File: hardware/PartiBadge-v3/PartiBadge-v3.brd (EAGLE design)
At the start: 118.9 x 117.7 mm, 26 parts, among them J1 I2C, J2 Supply, T1 MMBT4401-7-F

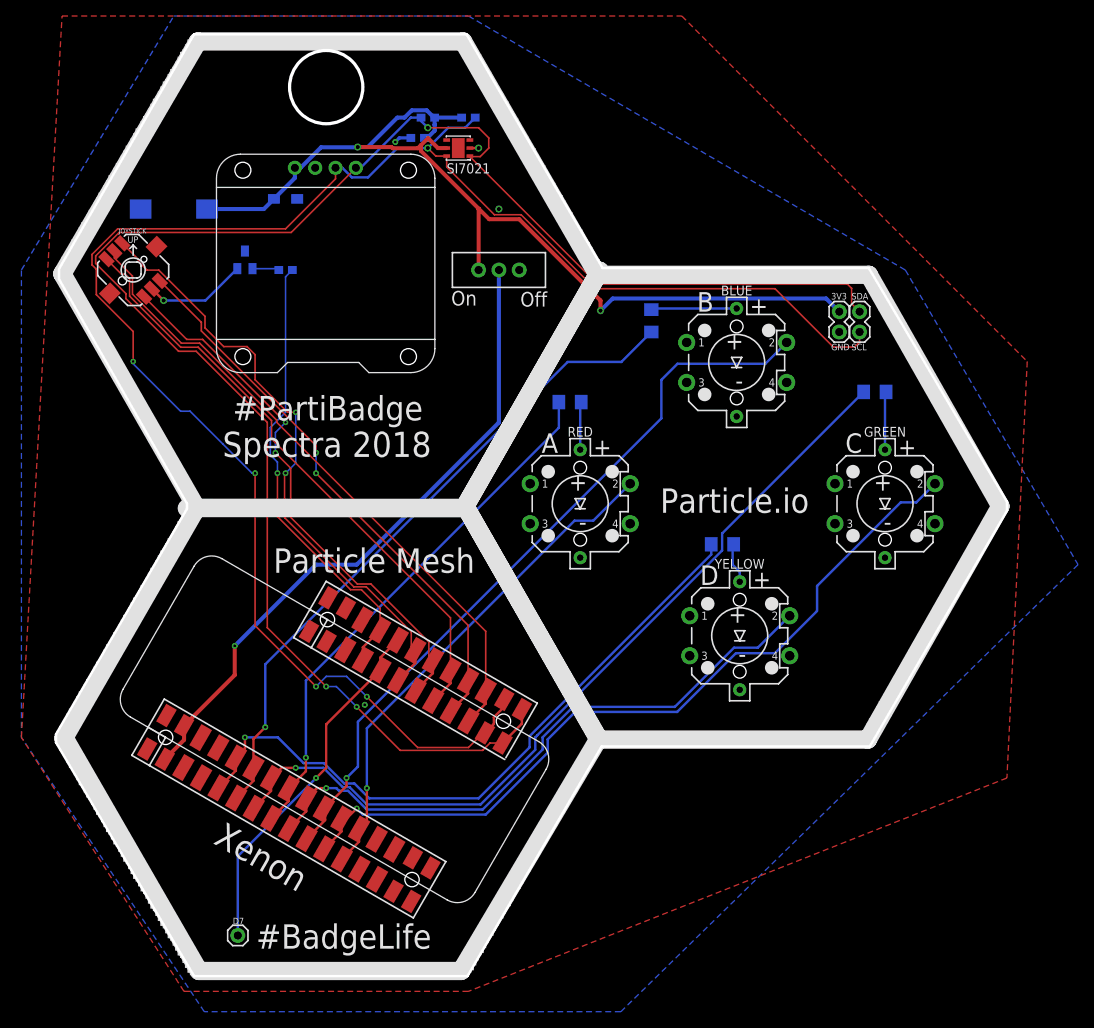
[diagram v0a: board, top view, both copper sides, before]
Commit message: finished Xenon port
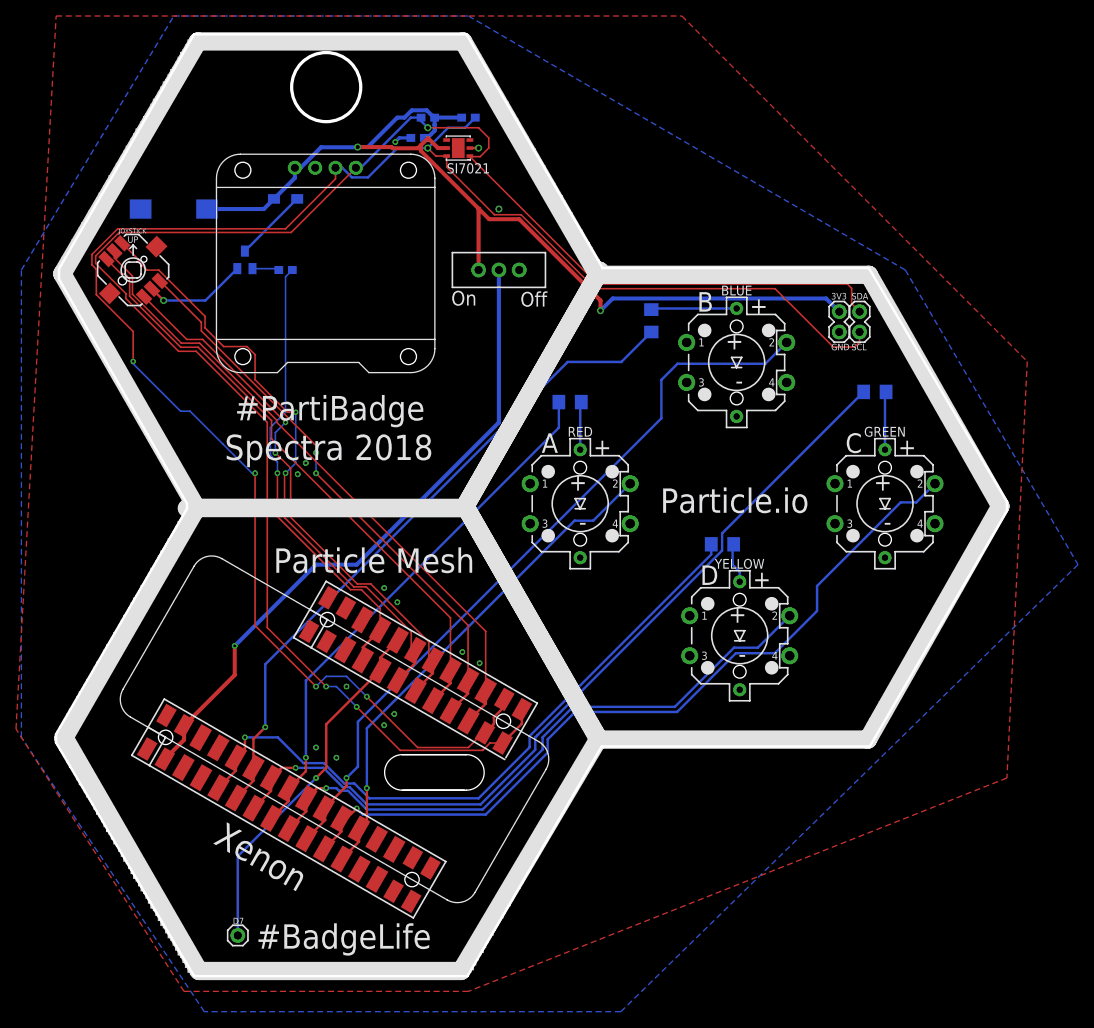
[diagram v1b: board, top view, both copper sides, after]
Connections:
- new net N$18: D1.A, T1.C
- net GND: no longer D1.A, T1.C
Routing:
- net N$18: track 0.00 -> 9.23 mm
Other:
- outline, holes or cut-outs redrawn
- board text added: "*NON PLATED * *SLOT*"
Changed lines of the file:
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@@
 <drawing>
 <settings>
-<setting alwaysvectorfont="no"/>
+<setting alwaysvectorfont="yes"/>
 <setting verticaltext="up"/>
 </settings>
-<grid distance="50" unitdist="mil" unit="mil" style="lines" multiple="1" display="no" altdistance="5" altunitdist="mil" altunit="mil"/>
+<grid distance="5" unitdist="mil" unit="mil" style="dots" multiple="1" display="yes" altdistance="5" altunitdist="mil" altunit="mil"/>
 <layers>
 <layer number="1" name="Top" color="4" fill="1" visible="yes" active="yes"/>
@@
 <layer number="26" name="bNames" color="7" fill="1" visible="yes" active="yes"/>
 <layer number="27" name="tValues" color="7" fill="1" visible="yes" active="yes"/>
-<layer number="28" name="bValues" color="7" fill="1" visible="yes" active="yes"/>
+<layer number="28" name="bValues" color="7" fill="1" visible="no" active="yes"/>
 <layer number="29" name="tStop" color="7" fill="3" visible="no" active="yes"/>
 <layer number="30" name="bStop" color="7" fill="6" visible="no" active="yes"/>
@@
 <layer number="45" name="Holes" color="7" fill="1" visible="yes" active="yes"/>
 <layer number="46" name="Milling" color="3" fill="1" visible="no" active="yes"/>
-<layer number="47" name="Measures" color="7" fill="1" visible="no" active="yes"/>
+<layer number="47" name="Measures" color="7" fill="1" visible="yes" active="yes"/>
 <layer number="48" name="Document" color="7" fill="1" visible="yes" active="yes"/>
 <layer number="49" name="Reference" color="7" fill="1" visible="yes" active="yes"/>
@@
 <wire x1="4.318" y1="33.401" x2="20.701" y2="61.595" width="0.3048" layer="20"/>
 <wire x1="20.701" y1="61.595" x2="20.701" y2="62.23" width="0.3048" layer="20"/>
-<text x="26.416" y="72.644" size="3.048" layer="21" font="vector" ratio="18">#PartiBadge</text>
-<text x="25.146" y="68.072" size="3.1496" layer="21" font="vector" ratio="18">Spectra 2018</text>
-<circle x="38.1" y="114.3" radius="4.57905" width="0.4064" layer="20"/>
+<text x="26.67" y="72.644" size="3.048" layer="21" font="vector" ratio="18">#PartiBadge</text>
+<text x="25.4" y="67.691" size="3.1496" layer="21" font="vector" ratio="18">Spectra 2018</text>
+<circle x="38.1" y="114.3" radius="4.318" width="0.4064" layer="20"/>
 <text x="65.024" y="68.58" size="2.4384" layer="21" font="vector" ratio="18">A</text>
 <text x="84.455" y="86.233" size="2.4384" layer="21" font="vector" ratio="18">B</text>
@@
 <rectangle x1="119.3546" y1="103.5812" x2="157.4546" y2="106.1212" layer="49"/>
 <rectangle x1="119.3546" y1="98.5012" x2="157.4546" y2="101.0412" layer="49"/>
-<dimension x1="2.54" y1="57.15" x2="104.14" y2="57.15" x3="53.34" y3="132.334" textsize="1.778" layer="47" dtype="diameter" unit="inch" visible="yes"/>
-<dimension x1="48.76095" y1="101.6" x2="57.91905" y2="101.6" x3="53.34" y3="124.46" textsize="1.778" layer="47" dtype="diameter" unit="inch" visible="yes"/>
 <dimension x1="51.689" y1="83.058" x2="64.008" y2="83.058" x3="57.8485" y3="111.125" textsize="1.778" layer="47" visible="yes"/>
-<dimension x1="61.71543125" y1="83.057990625" x2="61.72856875" y2="78.486009375" x3="105.918" y3="80.898996875" textsize="1.778" layer="47" dtype="diameter" visible="yes"/>
 <text x="23.876" y="19.812" size="3.1496" layer="21" font="vector" ratio="18" rot="R330">Xenon</text>
 <text x="31.496" y="53.594" size="3.048" layer="21" font="vector" ratio="18">Particle Mesh</text>
+<wire x1="47.625" y1="30.861" x2="55.499" y2="30.861" width="0.1524" layer="20"/>
+<wire x1="47.752" y1="26.416" x2="55.372" y2="26.416" width="0.1524" layer="20"/>
+<wire x1="55.499" y1="30.861" x2="55.626" y2="30.861" width="0.1524" layer="20"/>
+<wire x1="47.625" y1="30.861" x2="55.626" y2="30.861" width="0.1524" layer="20"/>
+<wire x1="55.626" y1="30.861" x2="55.626" y2="26.416" width="0.1524" layer="20" curve="-180"/>
+<wire x1="55.626" y1="26.416" x2="47.625" y2="26.416" width="0.1524" layer="20"/>
+<wire x1="47.625" y1="26.416" x2="47.625" y2="30.861" width="0.1524" layer="20" curve="-180"/>
+<text x="87.63" y="5.08" size="1.778" layer="48">*NON PLATED *
+*SLOT*</text>
+<wire x1="86.36" y1="7.62" x2="58.42" y2="25.4" width="0.1524" layer="48"/>
+<wire x1="58.42" y1="25.4" x2="59.69" y2="22.86" width="0.1524" layer="48"/>
+<wire x1="59.69" y1="22.86" x2="60.96" y2="25.4" width="0.1524" layer="48"/>
+<wire x1="60.96" y1="25.4" x2="58.42" y2="25.4" width="0.1524" layer="48"/>
+<dimension x1="47.625" y1="30.861" x2="47.625" y2="26.416" x3="115.951" y3="28.6385" textsize="1.778" layer="47" dtype="vertical"/>
 </plain>
 <attributes>
@@
 </polygon>
 <polygon width="0.3048" layer="1" isolate="0.3048">
-<vertex x="5.08" y="123.19"/>
+<vertex x="4.34483125" y="123.19"/>
 <vertex x="82.55" y="123.19"/>
 <vertex x="125.73" y="80.01"/>
@@
 <vertex x="55.88" y="1.27"/>
 <vertex x="20.32" y="1.27"/>
-<vertex x="0" y="33.02"/>
+<vertex x="-0.675690625" y="34.075765625"/>
 </polygon>
 <wire x1="16.321128125" y1="89.08886875" x2="17.779996875" y2="87.63" width="0.3048" layer="1"/>
@@
 <contactref element="MS1" pad="4'"/>
 <contactref element="MS1" pad="4"/>
-<contactref element="D1" pad="A"/>
 <contactref element="LS1" pad="2"/>
 <contactref element="T1" pad="E"/>
-<contactref element="T1" pad="C"/>
 <wire x1="17.78" y1="87.63" x2="23.01" y2="87.63" width="0.3048" layer="16"/>
 <wire x1="23.01" y1="87.63" x2="26.99" y2="91.61" width="0.3048" layer="16"/>
@@
 </signal>
 <signal name="N$2">
-<via x="42.926" y="37.084" extent="1-16" drill="0.35"/>
+<via x="35.56" y="67.31" extent="1-16" drill="0.35"/>
+</signal>
+<signal name="N$6">
+<via x="34.544" y="65.913" extent="1-16" drill="0.35"/>
+</signal>
+<signal name="N$9">
+<via x="45.339" y="51.689" extent="1-16" drill="0.35"/>
+</signal>
+<signal name="N$11">
+<via x="46.99" y="49.911" extent="1-16" drill="0.35"/>
+</signal>
+<signal name="N$12">
+<via x="55.118" y="43.688" extent="1-16" drill="0.35"/>
+</signal>
+<signal name="N$13">
+<via x="57.277" y="42.291" extent="1-16" drill="0.35"/>
+</signal>
+<signal name="N$14">
+<via x="45.339" y="34.544" extent="1-16" drill="0.35"/>
+</signal>
+<signal name="N$15">
+<via x="46.609" y="35.941" extent="1-16" drill="0.35"/>
+</signal>
+<signal name="N$16">
+<via x="39.37" y="30.48" extent="1-16" drill="0.35"/>
+</signal>
+<signal name="N$17">
+<via x="36.83" y="31.75" extent="1-16" drill="0.35"/>
+</signal>
+<signal name="N$18">
+<contactref element="D1" pad="A"/>
+<contactref element="T1" pad="C"/>
+<wire x1="27.94" y1="93.81" x2="34.46" y2="100.33" width="0.3048" layer="16"/>
+<wire x1="34.46" y1="100.33" x2="34.47" y2="100.33" width="0.3048" layer="16"/>
+</signal>
+<signal name="N$19">
+<via x="40.64" y="39.37" extent="1-16" drill="0.35"/>
 </signal>
 </signals>
@@
 </drawing>
 <compatibility>
+<note version="6.3" minversion="6.2.2" severity="warning">
+Since Version 6.2.2 text objects can contain more than one line,
+which will not be processed correctly with this version.
+</note>
 <note version="8.2" severity="warning">
 Since Version 8.2, EAGLE supports online libraries. The ids
